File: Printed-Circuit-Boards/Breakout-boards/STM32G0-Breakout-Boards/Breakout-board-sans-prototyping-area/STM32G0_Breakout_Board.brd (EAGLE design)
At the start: 19.7 x 21.6 mm, 13 parts, among them U1 STM32G0_SO8_T2

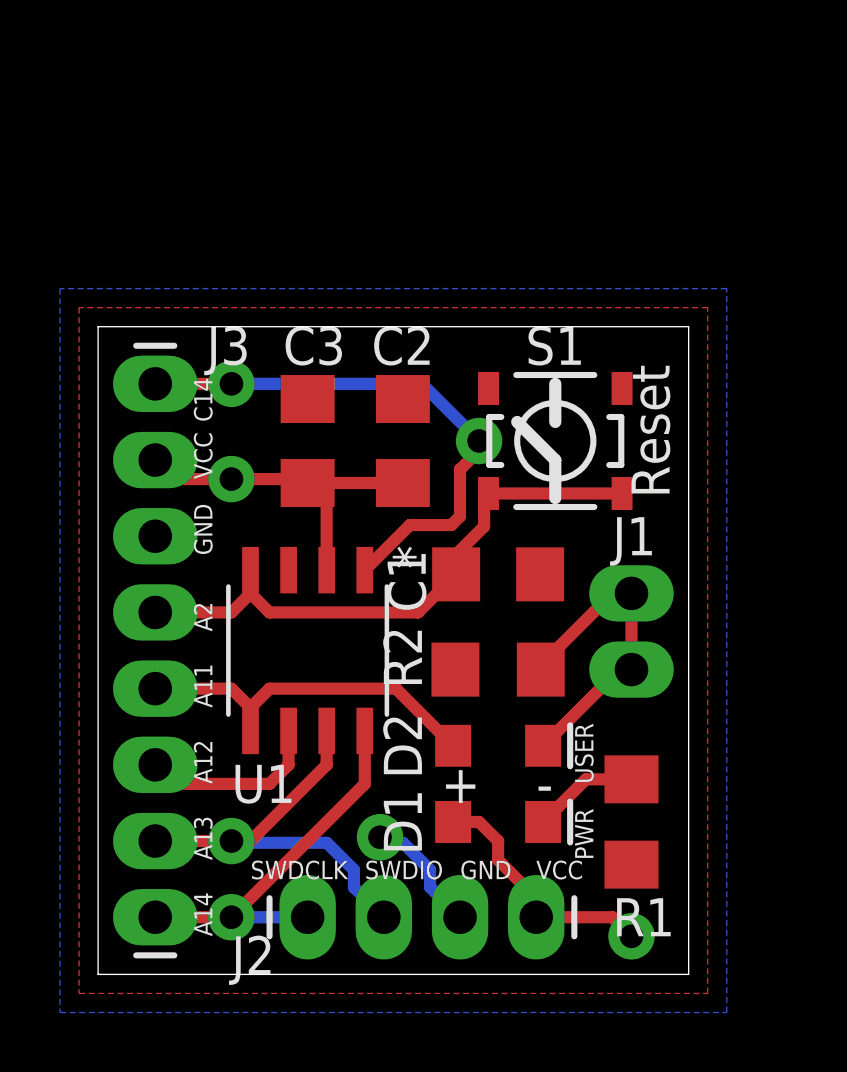
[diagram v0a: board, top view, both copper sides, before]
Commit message: Updated PCB files.
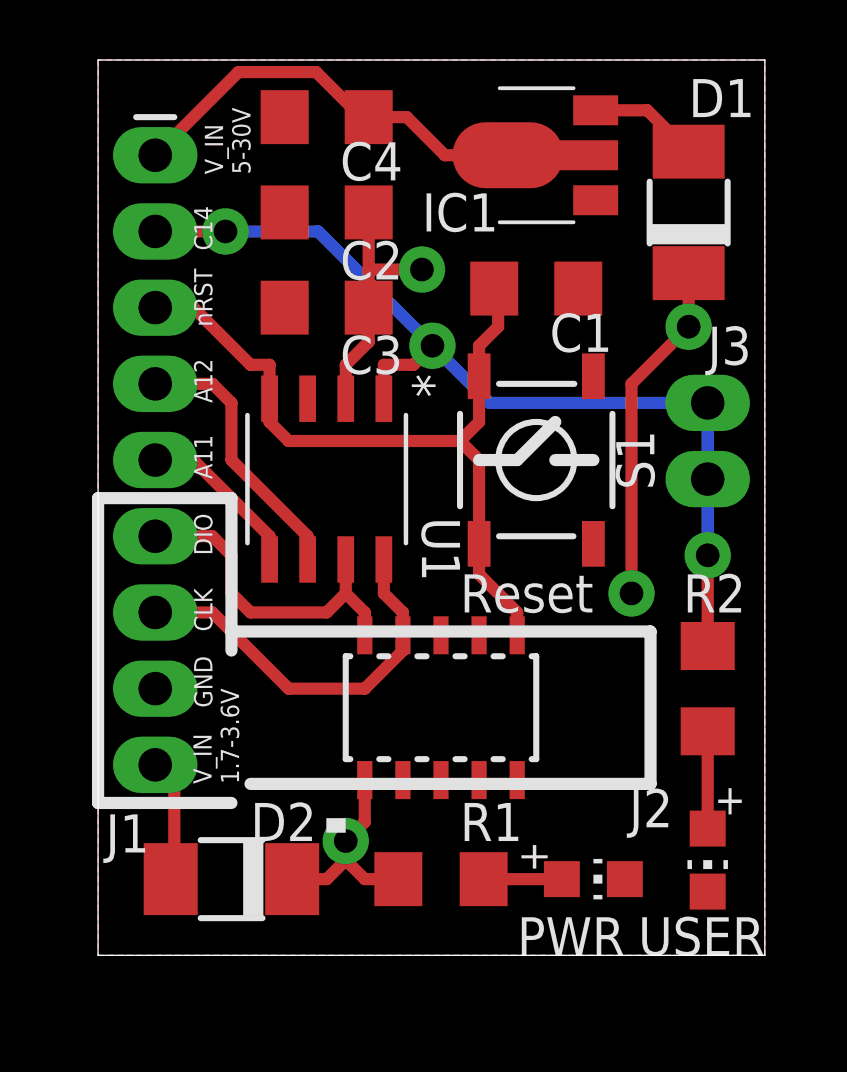
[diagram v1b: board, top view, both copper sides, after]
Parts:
- added C4: 10uF, adafruit:C1206
- added IC1: MCP170312MB, linear:SOT89
- added PWR, USER: (no value), adafruit:CHIP-LED0805
- D1, D2: device SparkFun-LED:LED-1206 -> diode:DO-214AC
- J1: device SparkFun-Connectors:1X02_LONGPADS -> SparkFun-Connectors:1X09_LONGPADS
- J2: value (none) -> CORTEX_DEBUG_SMD; device SparkFun-Connectors:1X04_LONGPADS -> SparkFun-Connectors:SAMTECH_FTSH-105-01
- J3: device SparkFun-Connectors:1X08_LONGPADS -> SparkFun-Connectors:1X02_LONGPADS
- R1, R2: value (none) -> 100
- S1: value MOMENTARY-SWITCH-SPST-SMD-4.5MM -> MOMENTARY-SWITCH-SPST-SMD-5.2-REDUNDANT; device SparkFun-Switches:TACTILE_SWITCH_SMD_4.5MM -> SparkFun-Switches:TACTILE_SWITCH_SMD_5.2MM
- moved D1 21.3 mm to (19.7, 24.8), turned to 90 degrees
- moved J3 18.7 mm to (20.3, 15.9), turned to 90 degrees
- moved J1 16.9 mm to (1.91, 6.35), turned to 90 degrees
- moved D2 9.94 mm to (4.45, 2.54), turned to 180 degrees
- moved C1 9.61 mm to (14.6, 22.2)
- moved FRAME1 8.98 mm to (0.00, 6.35)
- moved J2 8.28 mm to (11.4, 8.26)
- moved C2 8.03 mm to (7.62, 24.8), turned to 180 degrees
- moved R2 7.01 mm to (20.3, 8.89), turned to 90 degrees
- moved R1 6.63 mm to (11.4, 2.54), turned to 180 degrees
- moved U1 5.75 mm to (7.62, 15.9)
- moved C3 4.49 mm to (7.62, 21.6), turned to 180 degrees
- moved S1 0.90 mm to (14.6, 16.5), turned to 270 degrees
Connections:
- removed net N$11: D1.C, R1.1
- removed net PB7/PB8/PB9/PC14: J3.1, U1.1
- new net N$2: D2.A, J1.1
- new net N$3: C4.1, IC1.2@1, J1.9
- new net N$4: PWR.A, R1.1
- new net N$5: D1.A, IC1.3
- new net PC14: J1.8, J3.1, J3.2, R2.2, U1.1
- net GND: now also C4.2, IC1.1, J1.2, J2.5, J2.9, PWR.C, S1.1, USER.C; no longer J3.3, R1.2, R2.1, S1.3
- net N$1: now also R2.1, USER.A; no longer D2.C, J1.1, J1.2, R2.2
- net NRST/PA0/PA1/PA2: now also J1.7, J2.10, S1.3; no longer J3.4, S1.1
- net PA12: now also J1.6; no longer J3.6
- net PB0/PB1/PA8/PA11: now also J1.5; no longer D2.A, J3.5
- net SWDCLK: now also J1.3, J2.4; no longer J2.1, J3.8
- net SWDIO: now also J1.4; no longer J3.7
- net VCC: now also D1.C, D2.C, J2.1, R1.2; no longer D1.A, J2.4, J3.2
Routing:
- net PC14: track 0.00 -> 31.9 mm, vias 0 -> 3
- net PB7/PB8/PB9/PC14: track 18.3 -> 0.00 mm, vias 2 -> 0
- net N$3: track 0.00 -> 14.1 mm
- net N$1: track 10.7 -> 3.24 mm
- net VCC: track 19.7 -> 26.8 mm, vias 2 -> 4
- net NRST/PA0/PA1/PA2: track 19.4 -> 26.0 mm
- net PB0/PB1/PA8/PA11: track 12.0 -> 5.64 mm
- net N$2: track 0.00 -> 4.12 mm
- net GND: track 4.11 -> 0.00 mm, vias 1 -> 0
- net N$5: track 0.00 -> 3.67 mm
- net N$11: track 3.53 -> 0.00 mm
- net SWDIO: track 14.4 -> 11.2 mm, vias 1 -> 0
- net PA12: track 6.10 -> 9.07 mm
- net N$4: track 0.00 -> 2.61 mm
- net SWDCLK: vias 1 -> 0
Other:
- board size 19.7 x 21.6 mm -> 22.2 x 29.8 mm
- board text added: "."
- board text added: "CLK"
- board text added: "DIO"
- board text added: "V_IN 1.7-3.6V"
- board text added: "V_IN 5-30V"
- board text added: "V_IN, 1.7-3.6V: Connected thru D2 to V_DD; MCU damage may occur if >4V applied to this pin. V_IN, 5-30V: Connected to input of IC1 Max GPIO current, single pin: 15 mA Max GPIO current, all pins: 80 mA USER LED connected to C14 (pin 1). Cut trace btwn J3 pins on BOTTOM of PCB to remove LED from circuit (in- stall jumper on TOP to reinsert LED) ------------------------------ U1: STM32G031J6M6 / SOI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"
- board text added: "nRST"
- board text removed: "+"
- board text removed: "-"
- board text removed: "A13"
- board text removed: "A14"
- board text removed: "A2"
- board text removed: "PWR"
- board text removed: "SWDCLK"
- board text removed: "SWDIO"
- board text removed: "U1: STM32G031J6M6 | SOIC8 C1, C3: 100nF | 1206 C2: 4.7uF | 1206 S1: SPST-NO | 4.5mmx4.5mm R1, R2, D1, D2: 1206 ----------------- VCC: 1.7-3.6V (NOT REGULATED) D2 connected to B0/B1/A8/A11 Cut trace btwn terminals of J1 to rm D2 from circuit (can install jumper later) For more information: https://github.com/nathancharlesjones/ Embedded-for-Everyone"
- board text removed: "USER"
- board text removed: "VCC"
